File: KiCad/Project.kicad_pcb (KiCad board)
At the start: 2 copper layers, 132.9 x 81.5 mm, 44 parts, among them J2 Inputs Test Points, J3 Power & Output Test Points, Q1 BUK9832-55A, Q2 BUK9832-55A, SW1 Power, SW2 Fire, SW3 Freq Select, SW4 Fire Select, U1 TLV1117-50, U2 PIC16F1788-IP, U3 Audio Board

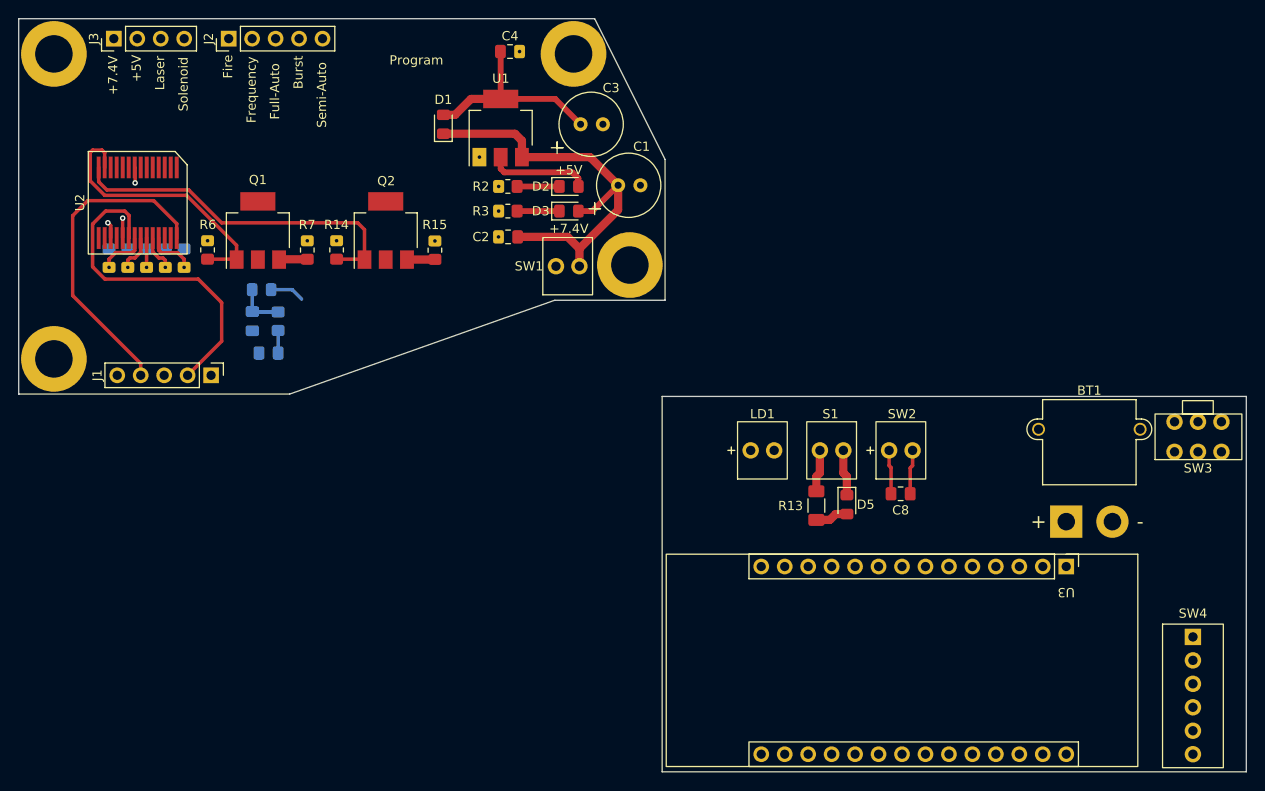
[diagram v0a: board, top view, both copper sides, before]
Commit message: blaster PCB is nearly finished
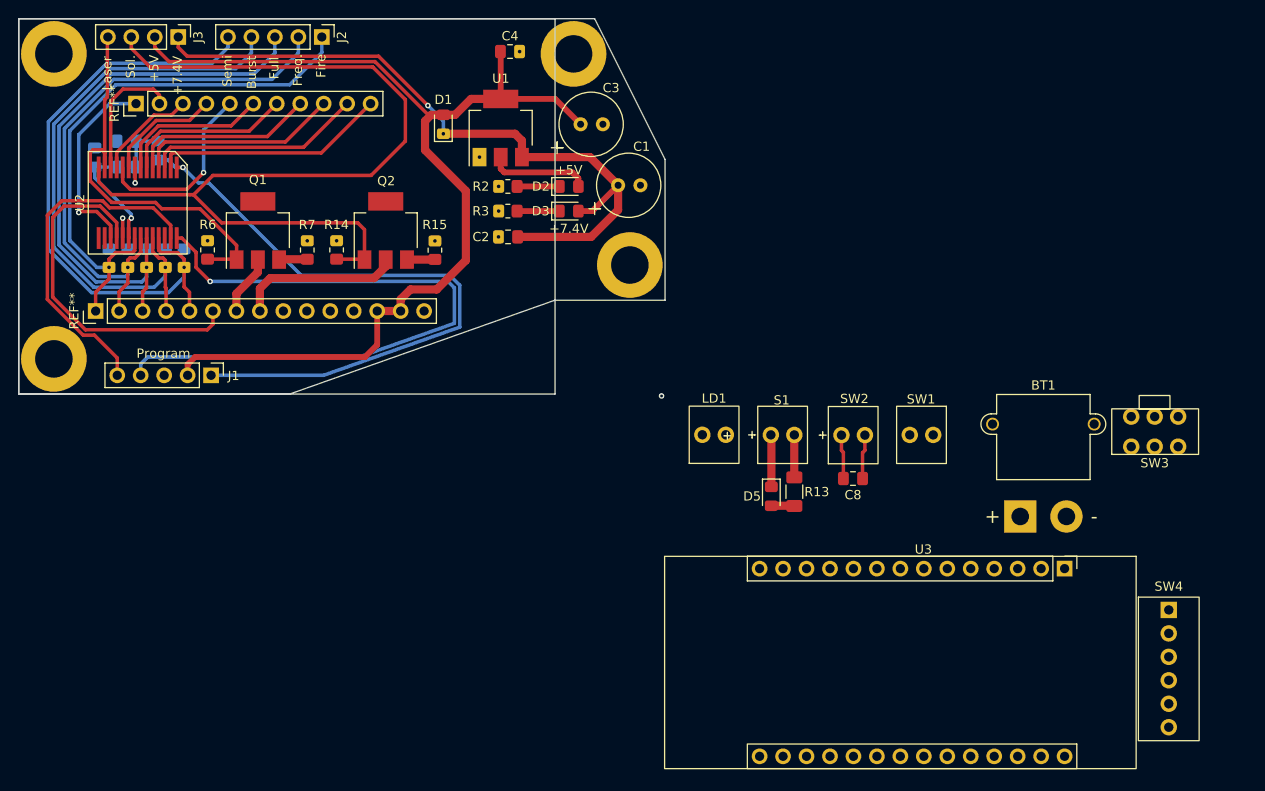
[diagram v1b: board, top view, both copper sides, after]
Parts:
- added REF**: PinHeader_1x15_P2.54mm_Vertical, Connector_PinHeader_2.54mm:PinHeader_1x15_P2.54mm_Vertical, F.Cu at (98.5, 50.7)
- added REF**: PinHeader_1x11_P2.54mm_Vertical, Connector_PinHeader_2.54mm:PinHeader_1x11_P2.54mm_Vertical, F.Cu at (102.9, 28.2)
- moved SW1 44.7 mm to (189.2, 64.1), turned to -90 degrees
- moved C6 28.3 mm to (98.4, 34.1), turned to -90 degrees
- moved C7 23.8 mm to (101.9, 32.3), turned to 180 degrees
- moved R5 23.4 mm to (101.8, 35.1), turned to 180 degrees
- moved D4 18.8 mm to (105.3, 33.3), turned to 90 degrees
- moved J2 10.1 mm to (123.0, 21.0), turned to -90 degrees
- moved D5 8.23 mm to (171.7, 70.8)
- moved S1 8.03 mm to (171.6, 64.1), turned to 90 degrees
- moved J3 6.98 mm to (107.4, 21.0), turned to -90 degrees
- moved LD1 5.50 mm to (164.2, 64.1)
- moved C8 5.42 mm to (180.5, 68.8)
- moved SW2 5.42 mm to (179.2, 64.1)
- moved BT1 5.01 mm to (201.1, 59.2)
- moved SW3 4.72 mm to (210.6, 65.4)
- moved SW4 3.92 mm to (214.7, 83.1)
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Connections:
- BT1 pad : (no net) -> GND
- C6 pad 1: Net-(C6-Pad1) -> GND
- C7 pad 2: Net-(C7-Pad2) -> GND
- D5 pad 1: Net-(D5-K) -> +7.4V
- J1 pad 3: Net-(J1-Pad3) -> GND
- J2 pad 1: Fire -> Net-(U2-INT/AN12/RB0)
- J2 pad 2: Frequency Select -> Net-(SW3-A)
- J2 pad 3: Full-Auto -> Net-(U2-P1B/AN8/RB2)
- J2 pad 4: Burst -> Net-(U2-PGM/C12IN2-/AN8/RB3)
- J2 pad 5: Semi-Auto -> Net-(U2-P1D/AN11/RB4)
- J3 pad 1: +7.4V -> Net-(D1-K)
- J3 pad 3: Laser/PWM -> Net-(Q2-G)
- J3 pad 4: Solenoid -> Net-(Q1-G)
- R10 pad 2: Net-(R10-Pad2) -> GND
- R11 pad 2: Net-(R10-Pad2) -> GND
- R12 pad 2: Net-(R10-Pad2) -> GND
- R14 pad 2: Net-(R14-Pad2) -> GND
- R15 pad 2: Net-(R15-Pad2) -> GND
- R6 pad 2: Net-(R6-Pad2) -> GND
- R7 pad 2: Net-(R7-Pad2) -> GND
- R8 pad 2: Net-(R10-Pad2) -> GND
- R9 pad 2: Net-(R10-Pad2) -> GND
- S1 pad 1: Net-(D5-K) -> +7.4V
- U3 pad 14: Net-(U3-GND-Pad14) -> GND
- U3 pad 15: Net-(U3-GND-Pad14) -> GND
- U3 pad 18: Net-(U3-GND-Pad14) -> GND
- U3 pad 27: Net-(U3-GND-Pad14) -> GND
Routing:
- net Net-(D4-K): track 3.72 -> 71.3 mm, vias 0 -> 1
- net +5V: track 77.3 -> 143.8 mm, vias 0 -> 1
- net Net-(Q2-G): track 38.8 -> 101.8 mm
- net Net-(U2-P1D/AN11/RB4): track 5.36 -> 66.4 mm
- net Net-(U2-PGM/C12IN2-/AN8/RB3): track 4.00 -> 63.7 mm
- net Net-(U2-P1B/AN8/RB2): track 3.18 -> 61.7 mm
- net Net-(SW3-A): track 4.07 -> 61.2 mm
- net Net-(U2-INT/AN12/RB0): track 10.2 -> 65.3 mm
- net VOL+: track 0.00 -> 39.0 mm
- net RB7: track 34.9 -> 73.3 mm, vias 0 -> 1
- net RB6: track 0.00 -> 37.7 mm
- net Net-(D1-K): track 45.5 -> 77.0 mm, vias 0 -> 1
- net TRIG0: track 0.00 -> 25.3 mm
- net TRIG1: track 0.00 -> 23.5 mm
- net TRIG2: track 0.00 -> 21.9 mm
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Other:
- board size 132.9 x 81.5 mm -> 70 x 40.6 mm
- board text added: "Freq."
- board text added: "Full"
- board text added: "Semi"
- board text added: "Sol."
- board text removed: "Frequency"
- board text removed: "Full-Auto"
- board text removed: "Semi-Auto"
- board text removed: "Solenoid"
